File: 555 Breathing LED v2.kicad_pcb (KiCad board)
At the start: 2 copper layers, 74.9 x 31.8 mm, 14 parts, among them Q1 PN2222A, U1 LMC555xN

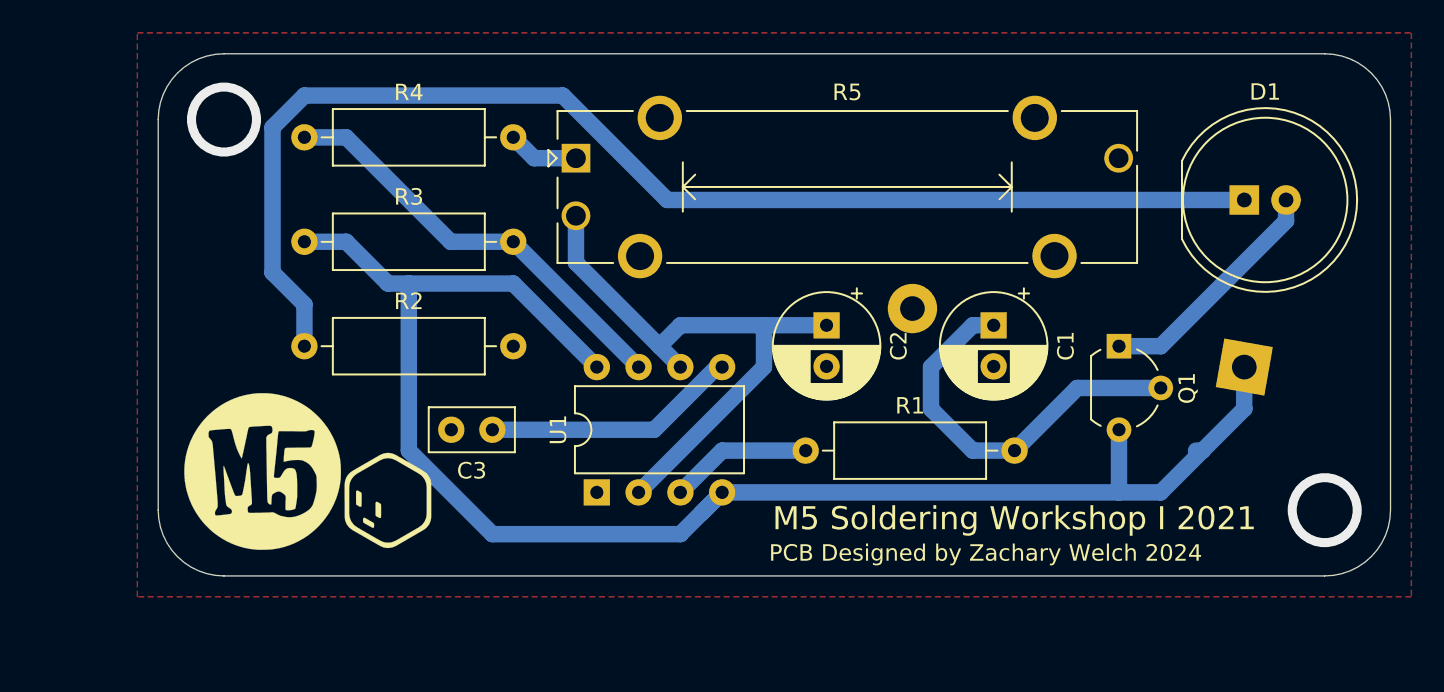
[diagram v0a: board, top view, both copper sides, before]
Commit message: Finished PCB
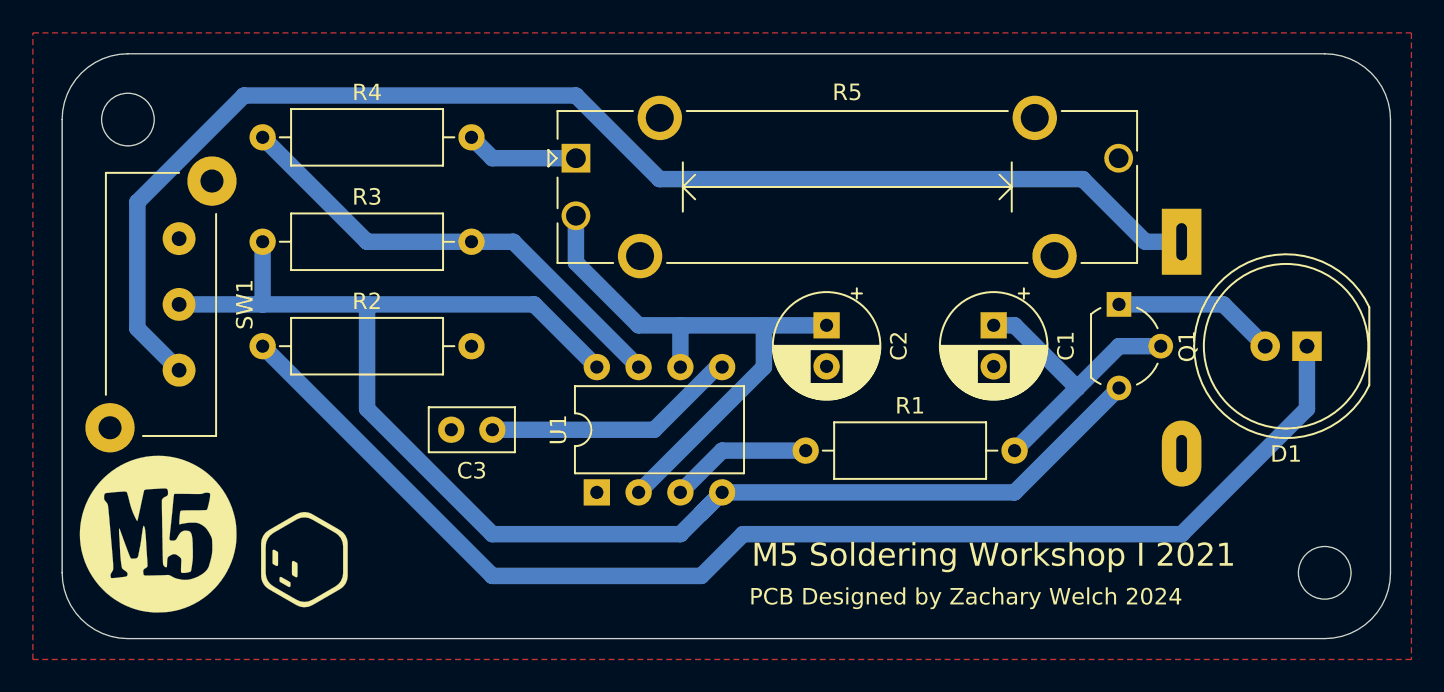
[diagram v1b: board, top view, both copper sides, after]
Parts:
- added REF**: MountingHole_3.2mm_M3, MountingHole:MountingHole_3.2mm_M3, F.Cu at (64.8, 69.8)
- added REF**: MountingHole_3.2mm_M3, MountingHole:MountingHole_3.2mm_M3, F.Cu at (130.8, 97.8)
- added SW1: SW_SPDT, 555-Breathing-LED-v2:MHS12204_SPDT, F.Cu at (61.0, 81.3)
- BT1: footprint Battery:BatteryHolder_Keystone_107_1x23mm -> 555-Breathing-LED-v2:BatteryHolder_MPD_BA9VPC_1xPP3noholes
- moved D1 9.67 mm to (129.5, 83.8), turned to 180 degrees
- moved BT1 8.52 mm to (121.9, 77.5), turned to 180 degrees
- moved ? 7.41 mm to (59.7, 95.2)
- moved ? 6.23 mm to (68.6, 96.8)
- moved Q1 2.54 mm to (118.1, 81.3)
- moved R2 2.54 mm to (66.0, 83.8)
- moved R3 2.54 mm to (66.0, 77.5)
- moved R4 2.54 mm to (66.0, 71.1)
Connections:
- BT1 pad 1: VCC -> Net-(BT1-Pad1)
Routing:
- net Net-(BT1-Pad1): track 0.00 -> 81.1 mm
- net Net-(C1-Pad1): track 24.0 -> 18.2 mm
- net Net-(D1-Pad2): track 14.6 -> 9.94 mm
- net VCC: track 95.7 -> 91.5 mm
- net Net-(R4-Pad2): track 4.34 -> 6.88 mm
- net Net-(R3-Pad2): track 26.1 -> 28.6 mm
- net Net-(D1-Pad1): track 76.7 -> 77.3 mm
- net (no net): vias 2 -> 0
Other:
- board size 74.9 x 31.8 mm -> 80.8 x 35.6 mm
